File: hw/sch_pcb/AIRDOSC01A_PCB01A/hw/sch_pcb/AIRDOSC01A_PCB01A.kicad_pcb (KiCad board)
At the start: 2 copper layers, 30 x 40.1 mm, 39 parts, among them J1 HEADER_2x01_PARALLEL, J10 HEADER_2x01_PARALLEL, J2 HEADER_2x01_PARALLEL, J3 HEADER_2x01_PARALLEL, J4 HEADER_2x01_PARALLEL, J5 HEADER_2x01_PARALLEL, J6 HEADER_2x01_PARALLEL, J7 HEADER_2x01_PARALLEL, J8 HEADER_2x01_PARALLEL, J9 HEADER_2x01_PARALLEL, M1 HOLE, M2 HOLE, M3 HOLE, M4 HOLE, U1 MICROFC-60035-SMT-TR(1), U2 OPA836IDB

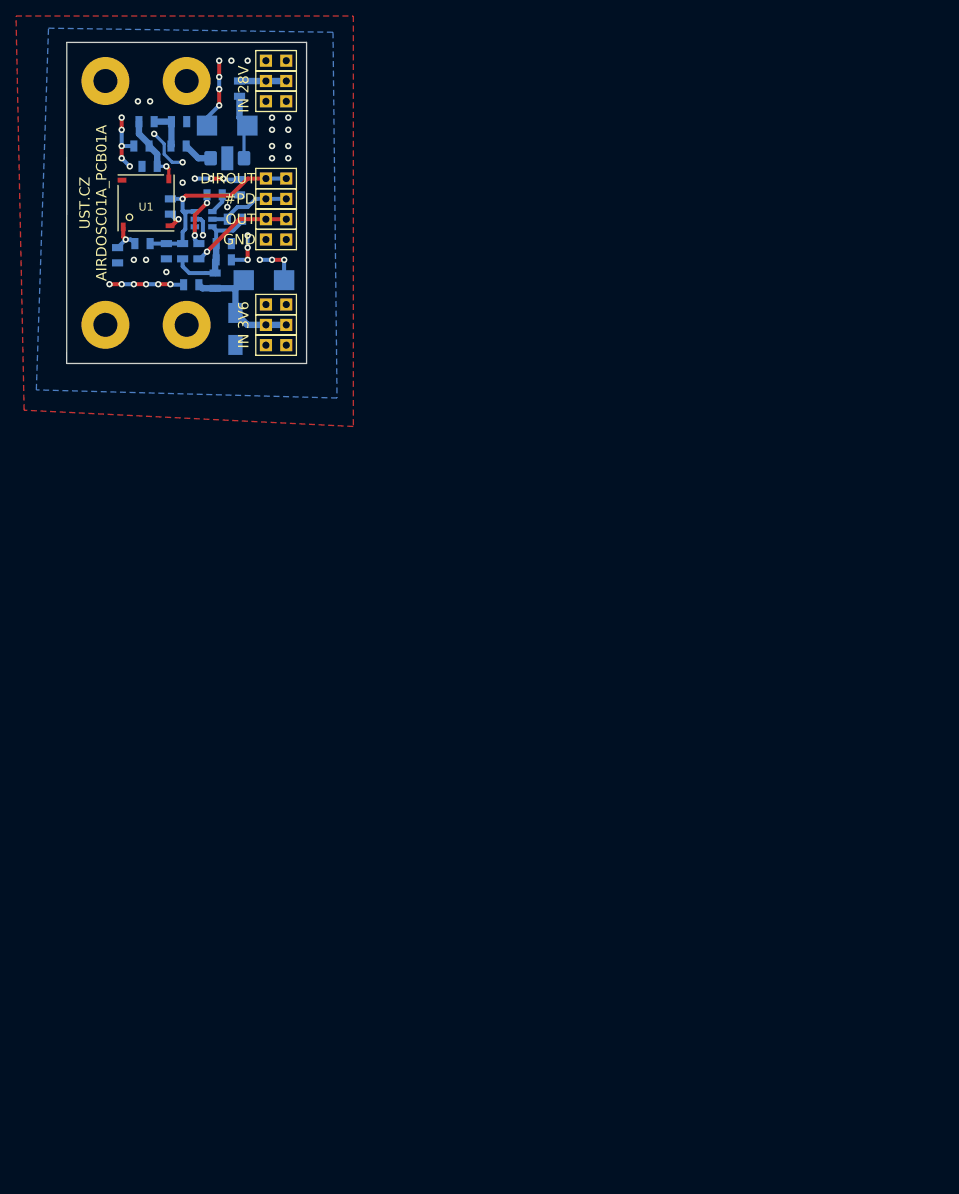
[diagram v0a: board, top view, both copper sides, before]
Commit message: Edit
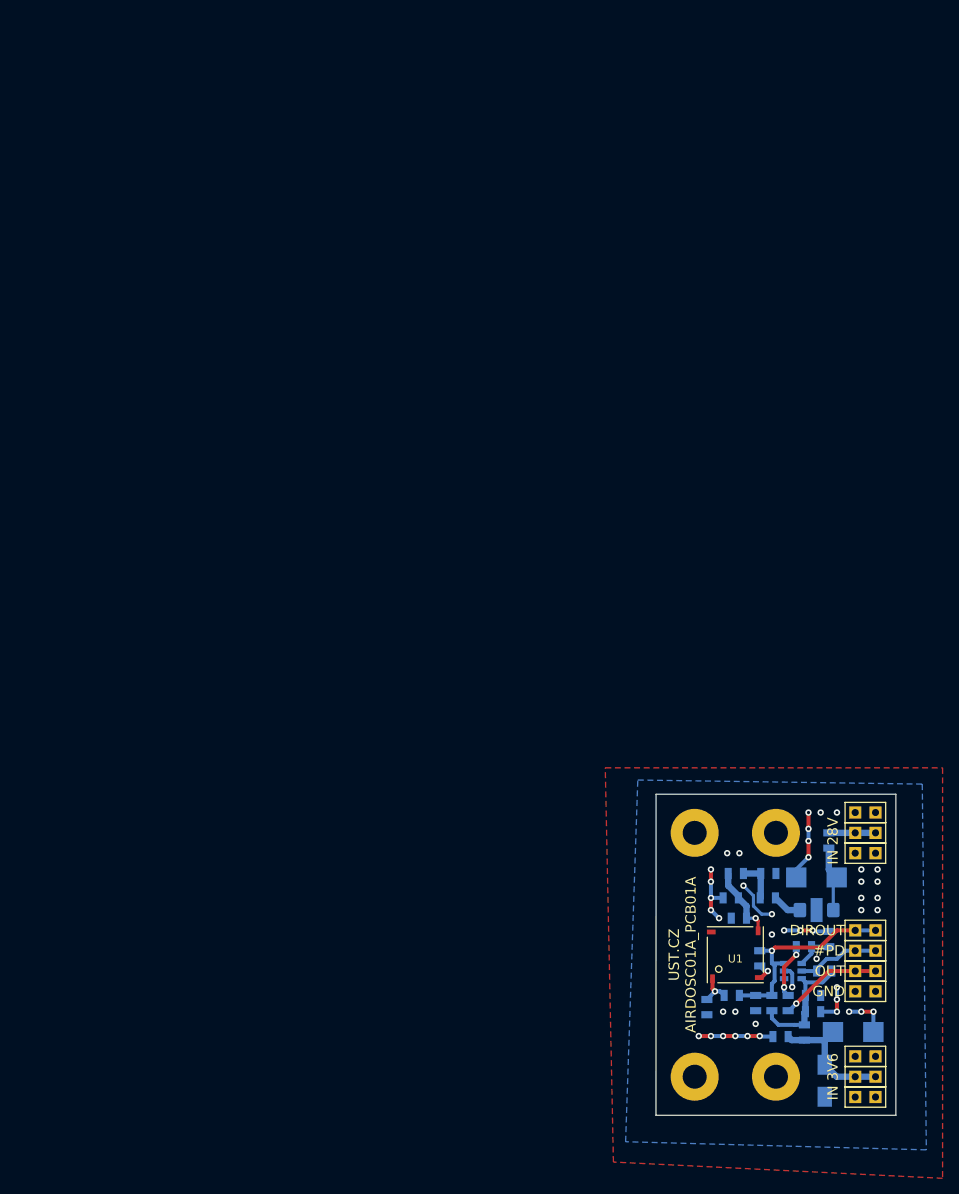
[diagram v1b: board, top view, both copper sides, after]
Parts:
- moved C2 119.4 mm to (94.0, 68.1)
- moved C3 119.4 mm to (98.6, 83.3)
- moved C4 119.4 mm to (89.5, 83.9)
- moved C5 119.4 mm to (87.9, 63.5)
- moved C6 119.4 mm to (83.2, 66.5)
- moved C7 119.4 mm to (93.5, 80.8)
- moved D1 119.4 mm to (95.0, 89.4)
- moved J1 119.4 mm to (100.1, 61.0)
- moved J10 119.4 mm to (100.1, 73.2)
- moved J2 119.4 mm to (100.1, 58.4)
- moved J3 119.4 mm to (100.1, 55.9)
- moved J4 119.4 mm to (100.1, 91.4)
- moved J5 119.4 mm to (100.1, 88.9)
- moved J6 119.4 mm to (100.1, 86.4)
- moved J9 119.4 mm to (100.1, 78.2)
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
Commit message: edit
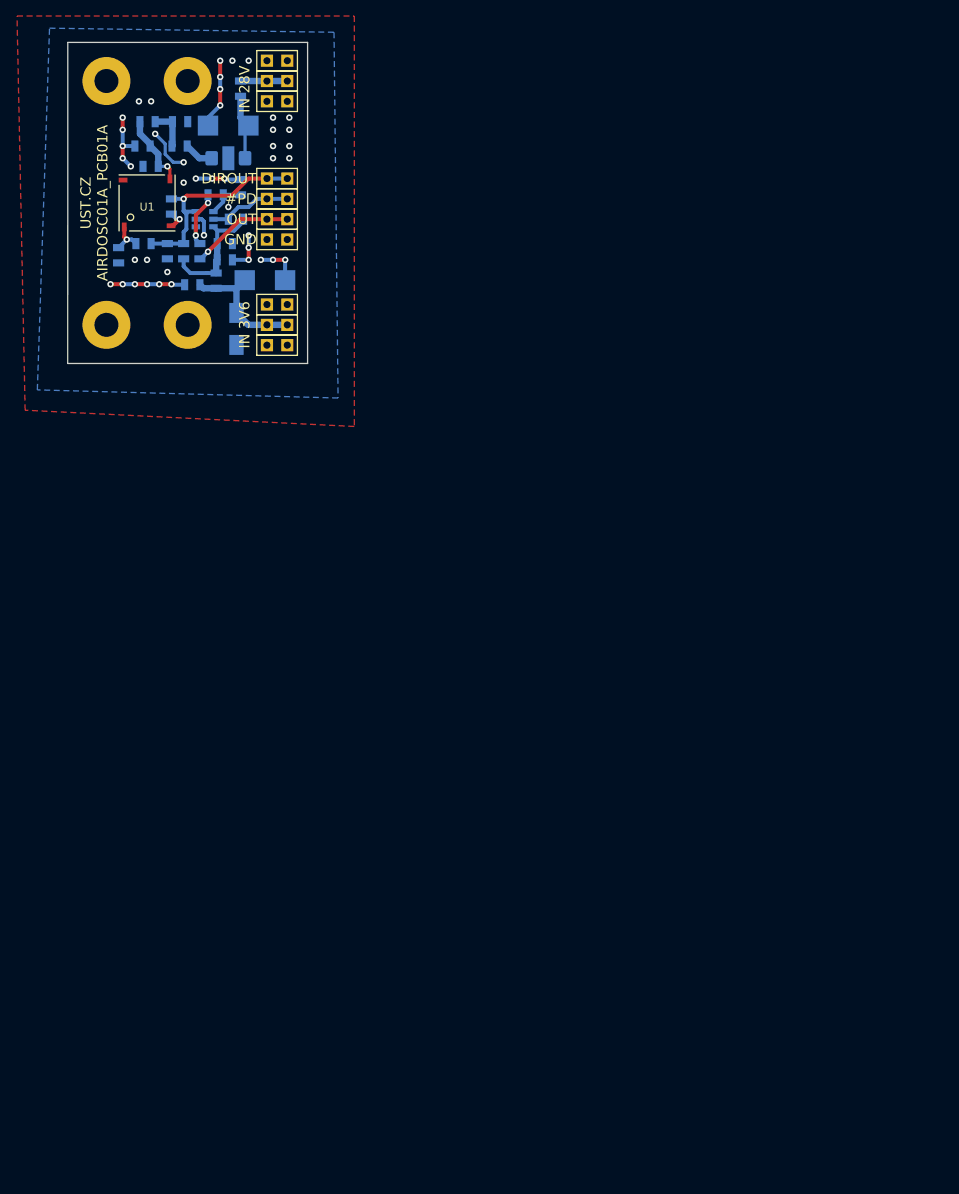
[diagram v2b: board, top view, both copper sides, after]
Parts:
- moved C1 119.3 mm to (20.4, -30.0)
- moved C10 119.3 mm to (9.84, -15.2)
- moved C2 119.3 mm to (20.4, -25.9)
- moved C3 119.3 mm to (25.0, -10.7)
- moved C4 119.3 mm to (15.9, -10.1)
- moved C5 119.3 mm to (14.4, -30.5)
- moved C6 119.3 mm to (9.72, -27.4)
- moved C7 119.3 mm to (20.0, -13.2)
- moved C8 119.3 mm to (20.0, -15.2)
- moved C9 119.3 mm to (10.7, -24.9)
- moved D1 119.3 mm to (21.5, -4.57)
- moved J1 119.3 mm to (26.5, -33.0)
- moved J10 119.3 mm to (26.5, -20.8)
- moved J2 119.3 mm to (26.5, -35.6)
- moved J3 119.3 mm to (26.5, -38.1)
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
